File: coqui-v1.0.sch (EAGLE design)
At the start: 33 parts, among them IC1 OPAMP-DUALU, IC2 OPAMP-DUALU, IC3 MCP73831, IC4 MCP1700-33, J1 AYZ0202, X1 USBSMD

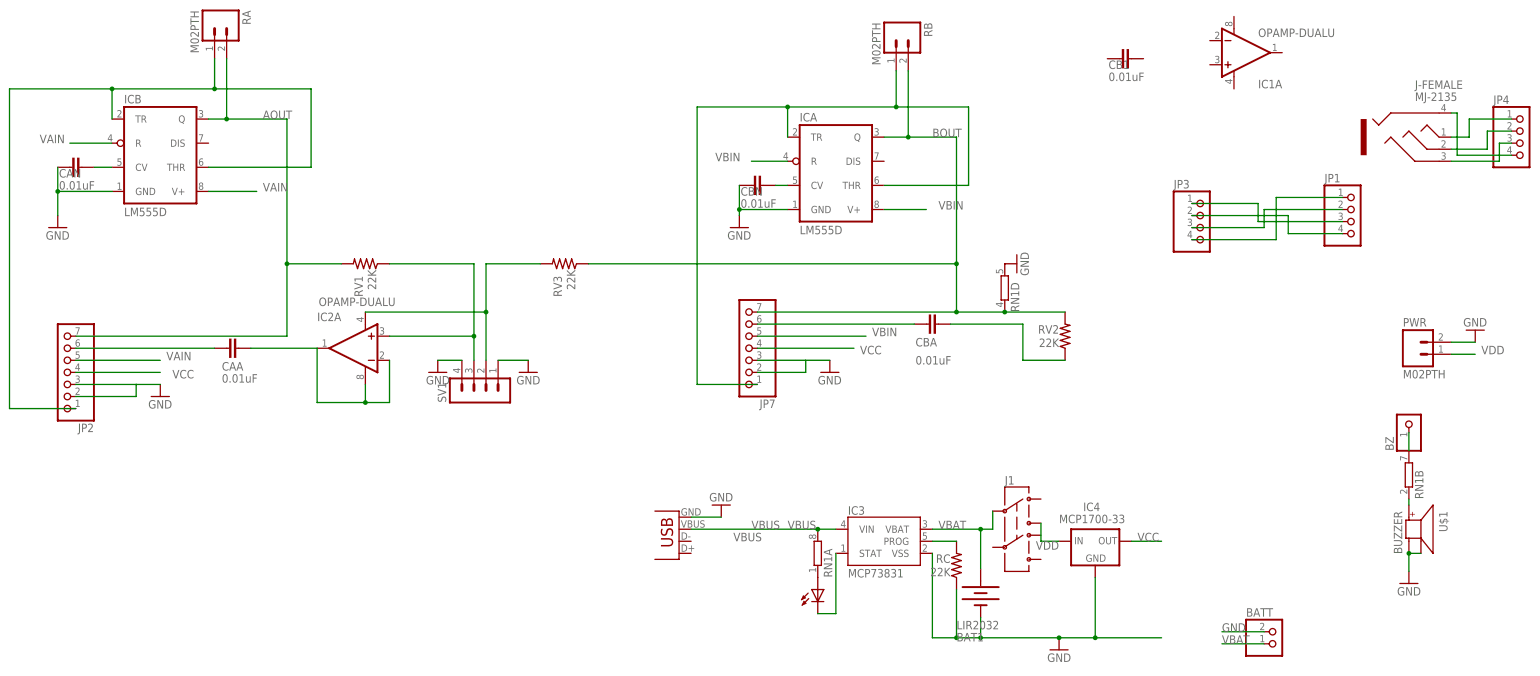
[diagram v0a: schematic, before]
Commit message: update
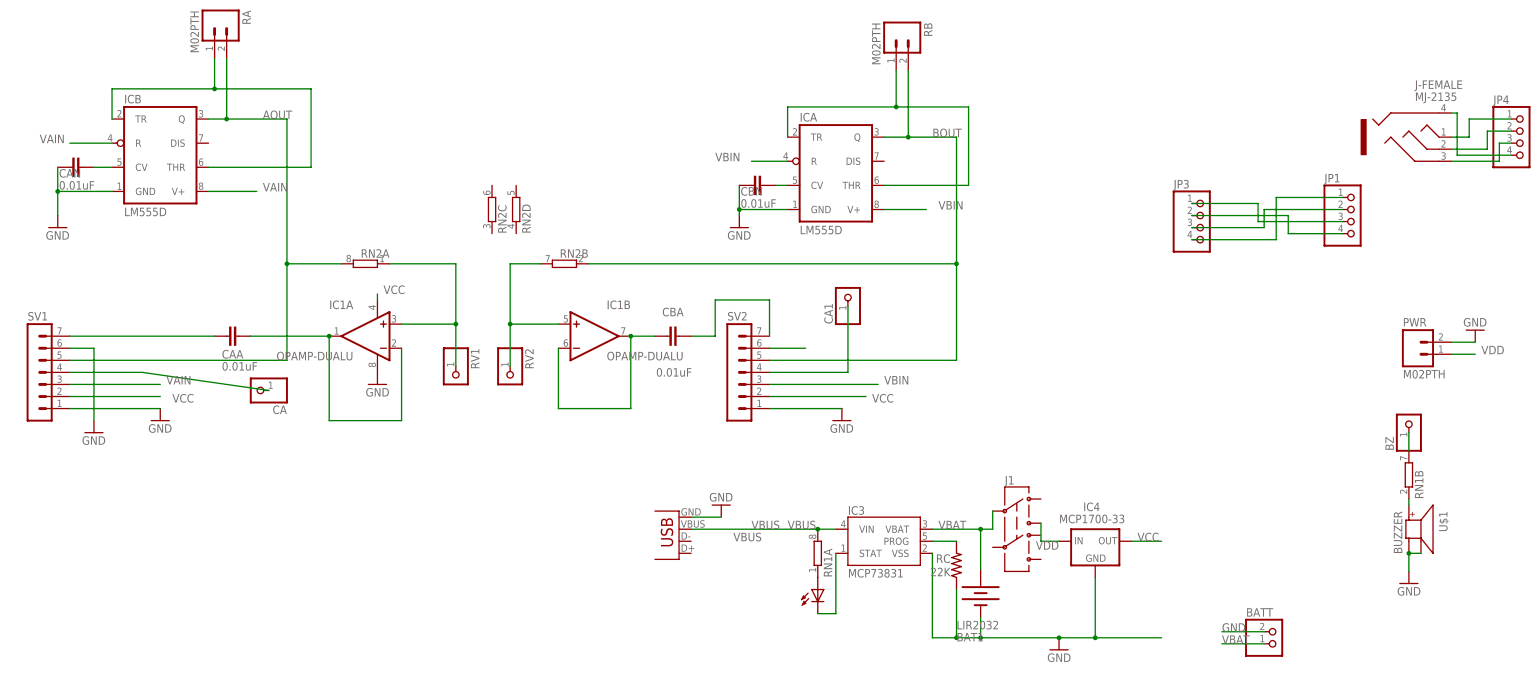
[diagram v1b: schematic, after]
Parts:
- removed CB1: 0.01uF, rcl:C-EUC0805
- removed IC2: OPAMP-DUALU, SparkFun-AnalogIC:OPAMP-DUALU
- removed JP2, JP7: (no value), pinhead:PINHD-1X7
- removed RV3: 22K, adafruit2013:R-US_R0805
- added CA, CA1: (no value), pinhead:PINHD-1X1
- added RN2: (no value), resistor-dil:4R-NEXB38V
- added SV2: (no value), con-lstb:MA07-1
- RV1, RV2: value 22K -> (none); device adafruit2013:R-US_R0805 -> pinhead:PINHD-1X1
- SV1: device con-lstb:MA04-1 -> con-lstb:MA07-1
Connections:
- removed net N$22: IC2A.V-, RV3.2, SV1.2
- new net N$24: CBA.1, IC1B.-IN, IC1B.OUT
- new net N$25: CA.1, SV1.4
- new net N$26: SV2.6
- new net N$27: CA1.1, SV2.4
- net AOUT: now also RN2A.2, SV1.5; no longer JP2.7, RV1.2
- net BOUT: now also RN2B.1, SV2.5; no longer JP7.7, RN1D.1, RV2.2, RV3.1
- net GND: now also IC1A.V+; no longer JP2.2, JP2.3, JP7.2, JP7.3, RN1D.2, SV1.4
- net N$10: now also IC1A.-IN, IC1A.OUT; no longer IC2A.-IN, IC2A.OUT, IC2A.V+
- net N$11: no longer JP2.1
- net N$13: now also SV2.7; no longer RV2.1
- net N$16: no longer JP7.1
- net N$17: now also SV1.6; no longer CBA.1, JP7.6
- net N$23: now also IC1A.+IN, IC1B.+IN, RN2A.1, RN2B.2; no longer IC2A.+IN, SV1.3
- net N$9: now also SV1.7; no longer JP2.6
- net VAIN: now also SV1.3; no longer JP2.5
- net VBIN: no longer JP7.5
- net VCC: now also IC1A.V-, SV1.2; no longer JP2.4, JP7.4
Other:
- moved on the sheet: CAA, CBA, IC1A
